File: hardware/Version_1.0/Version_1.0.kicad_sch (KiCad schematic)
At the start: 60 parts, among them J1 Conn_Coaxial, J2 Conn_Coaxial, J3 Conn_Coaxial, J4 Conn_Coaxial, J5 Conn_01x06_Pin, J6 Conn_01x06_Pin, J7 Conn_Coaxial, U1 ADF4351, Y1 SG-5032CAN

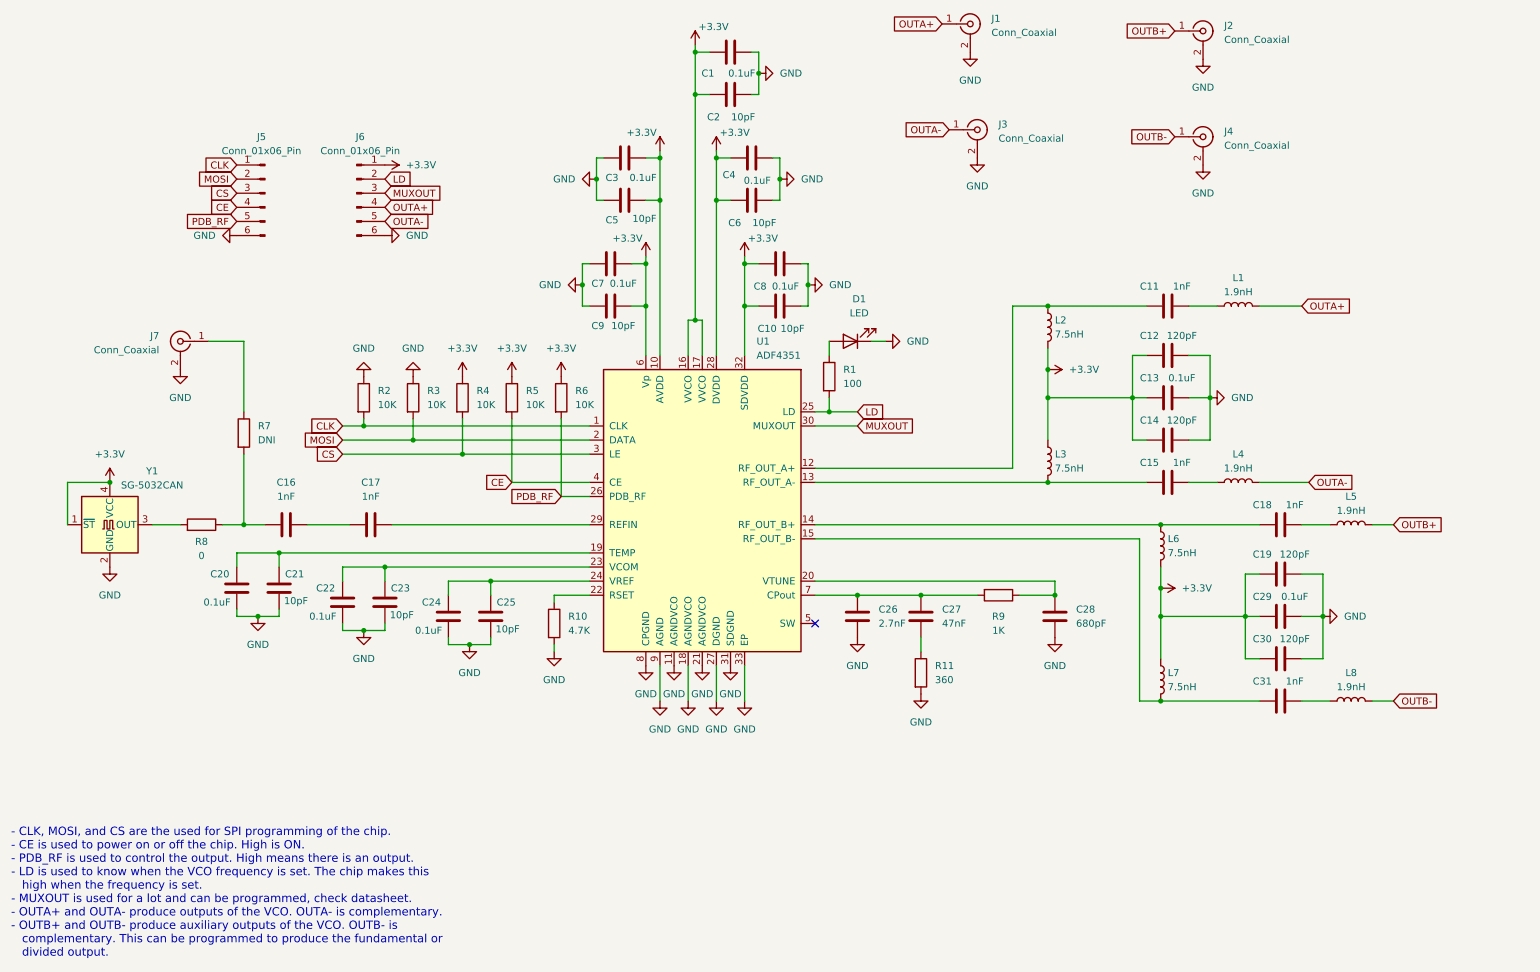
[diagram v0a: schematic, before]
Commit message: Finished v1 pcb
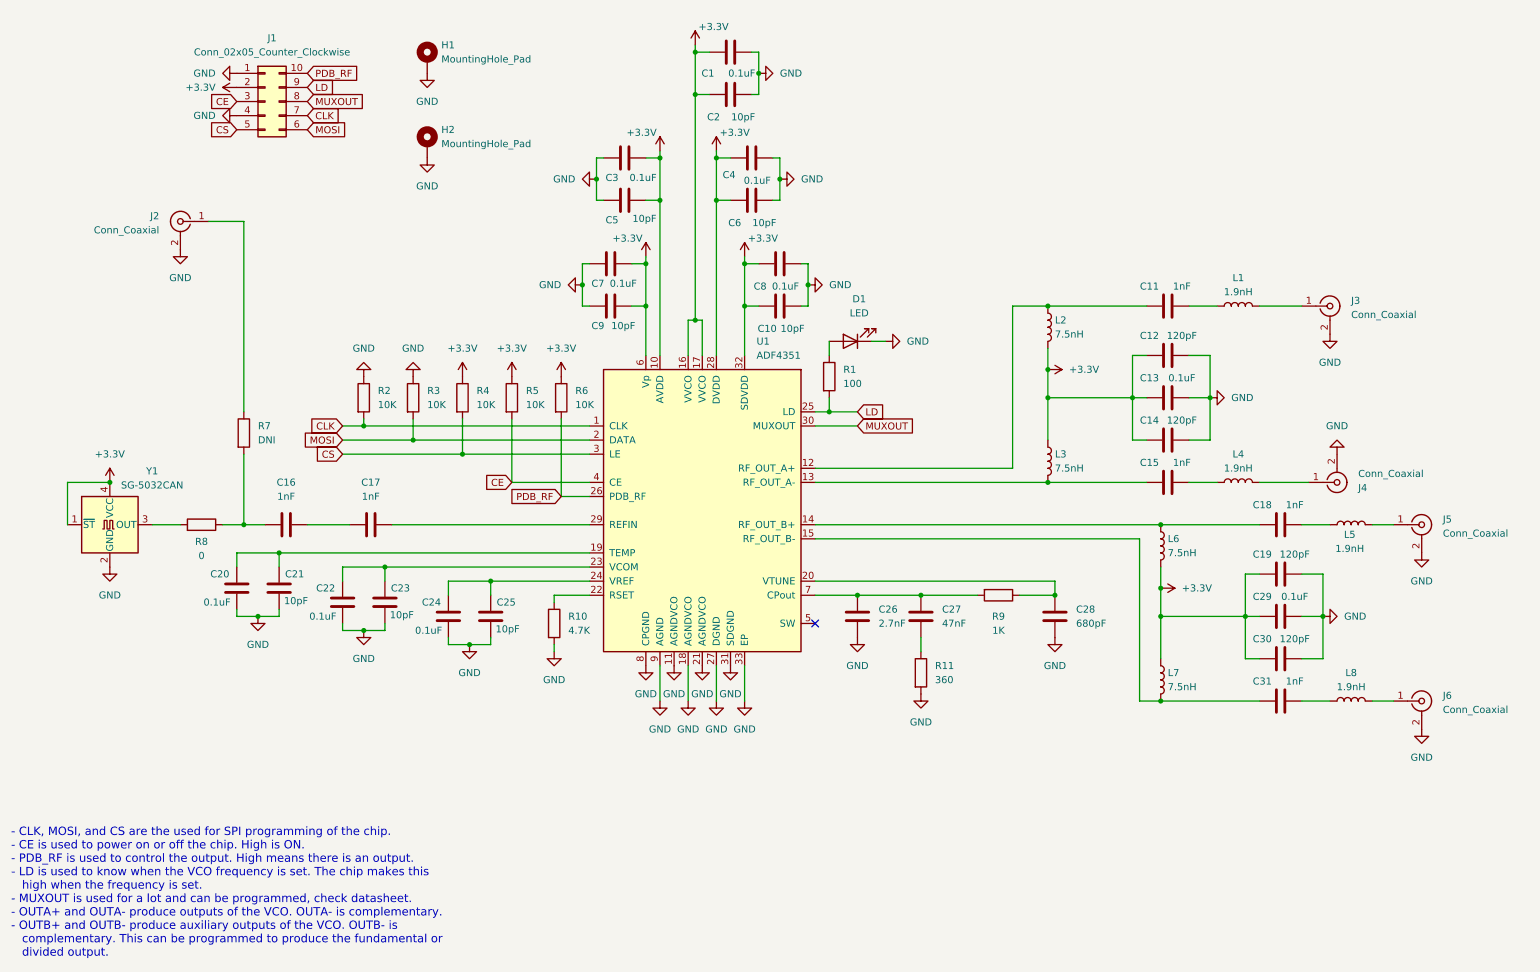
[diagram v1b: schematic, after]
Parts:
- removed J1, J2: Conn_Coaxial, Connector_Coaxial:SMA_Molex_73251-1153_EdgeMount_Horizontal, symbol Connector:Conn_Coaxial
- removed J5, J6: Conn_01x06_Pin, Connector_PinSocket_2.54mm:PinSocket_1x06_P2.54mm_Vertical, symbol Connector:Conn_01x06_Pin
- added H1, H2: MountingHole_Pad, MountingHole:MountingHole_3.2mm_M3_Pad, symbol Mechanical:MountingHole_Pad
- added J1: Conn_02x05_Counter_Clockwise, Connector_PinHeader_2.54mm:PinHeader_2x05_P2.54mm_Vertical, symbol Connector_Generic:Conn_02x05_Counter_Clockwise
- added J5, J6: Conn_Coaxial, Connector_Coaxial:SMA_Molex_73251-1153_EdgeMount_Horizontal, symbol Connector:Conn_Coaxial
- renumbered J7 to J2
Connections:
- net +3.3V: now also J1.2 (Pin_2)
- net CE: now also J1.3 (Pin_3)
- net CLK: now also J1.7 (Pin_7)
- net CS: now also J1.5 (Pin_5)
- net GND: now also H1.1, H2.1, J1.1 (Pin_1), J1.4 (Pin_4), J5.2 (Ext), J6.2 (Ext)
- net LD: now also J1.9 (Pin_9)
- net MOSI: now also J1.6 (Pin_6)
- net MUXOUT: now also J1.8 (Pin_8)
- net PDB_RF: now also J1.10 (Pin_10)
- net OUTA+: no longer names the net of L1.2
- net OUTA+: now also J3.1 (In)
- net OUTA-: no longer names the net of L4.2
- net OUTA-: now also J4.1 (In); no longer J3.1 (In)
- net OUTB+: no longer names the net of L5.2
- net OUTB+: now also J5.1 (In)
- net OUTB-: no longer names the net of L8.2
- net OUTB-: now also J6.1 (In); no longer J4.1 (In)
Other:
- moved on the sheet: J2
